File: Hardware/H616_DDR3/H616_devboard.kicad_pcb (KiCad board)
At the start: 8 copper layers, 50 x 50 mm, 169 parts, among them J1 Micro_SD_Card_Det2, J2 HDMI_D_1.4, J3 USB_C_Receptacle_USB2.0, J4 USB_C_Receptacle_USB2.0, J5 Conn_01x40_Pin, Q1 AO3420_C358680, Q2 AO3401A, Q3 AO3401A, SW1 CK_KMS2xxG, U1 H616, U10 D3V3XA4B10LP, U11 D3V3XA4B10LP, U2 K4B8G1646D, U3 AXP305, U4 SW6206, U6 KLMBG2JETD-B041, U7 AP6256, U8 D3V3XA4B10LP, U9 D3V3XA4B10LP, Y1 24MHz

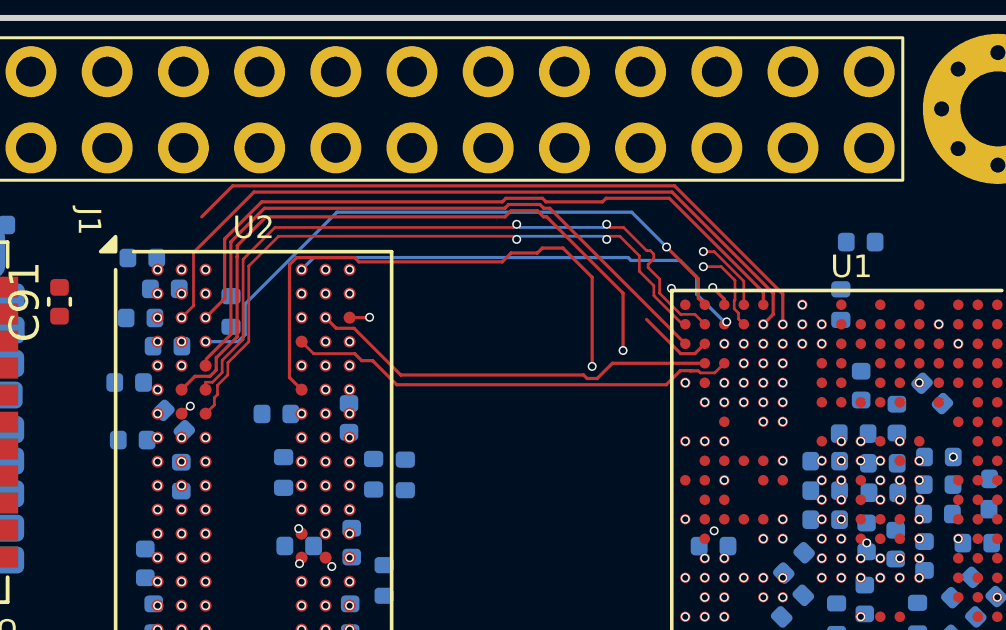
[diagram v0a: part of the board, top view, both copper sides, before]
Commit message: ddr trace
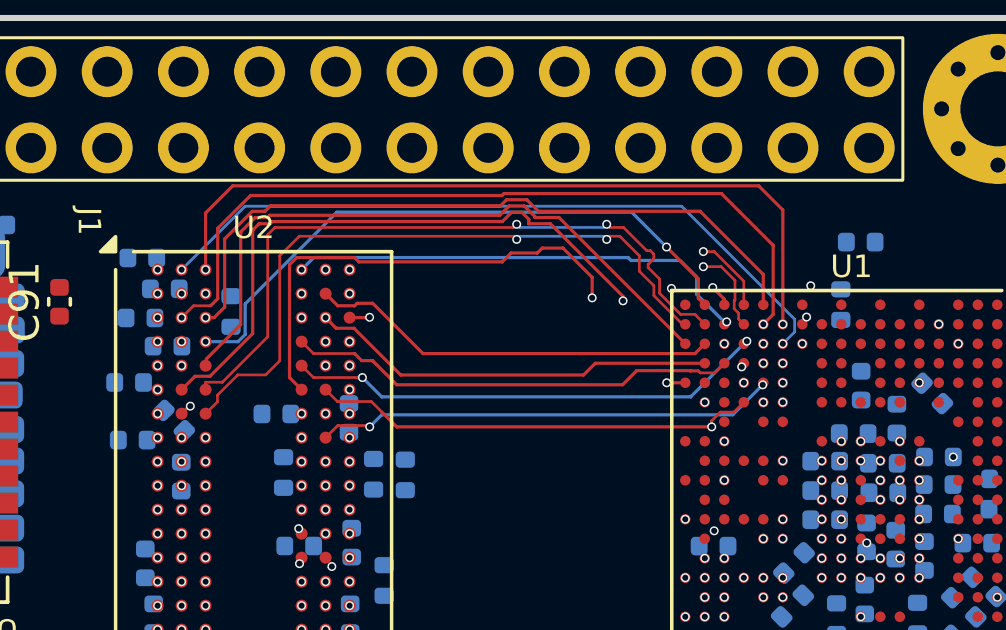
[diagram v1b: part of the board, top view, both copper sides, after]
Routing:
- net /DRAM/DQ6: track 0.39 -> 27.5 mm
- net /DRAM/DQ13: track 0.00 -> 23.9 mm
- net /DRAM/DQ4: track 0.00 -> 22.7 mm
- net /DRAM/DQ7: track 0.00 -> 20.0 mm
- net /DRAM/SDQM1: track 0.00 -> 16.0 mm
- net /DRAM/DQ5: track 0.00 -> 15.4 mm
- net /DRAM/DQ3: track 0.00 -> 14.9 mm, vias 2 -> 1
- net /DRAM/DQ14: track 2.55 -> 13.7 mm, vias 1 -> 0
- net /DRAM/DQ2: track 22.3 -> 26.6 mm
- net /DRAM/DQ15: track 22.3 -> 25.6 mm
- net /DRAM/DQ11: track 25.1 -> 26.3 mm
- net GND: track 2.07 -> 2.69 mm
- net /IO1/SDC0_D3: vias 1 -> 0
- net /IO1/SDC0_D2: vias 1 -> 0
- net /DRAM/SDQS2P: vias 1 -> 0
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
